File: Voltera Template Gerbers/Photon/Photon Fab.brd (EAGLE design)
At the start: 101.6 x 76.2 mm, 1 part

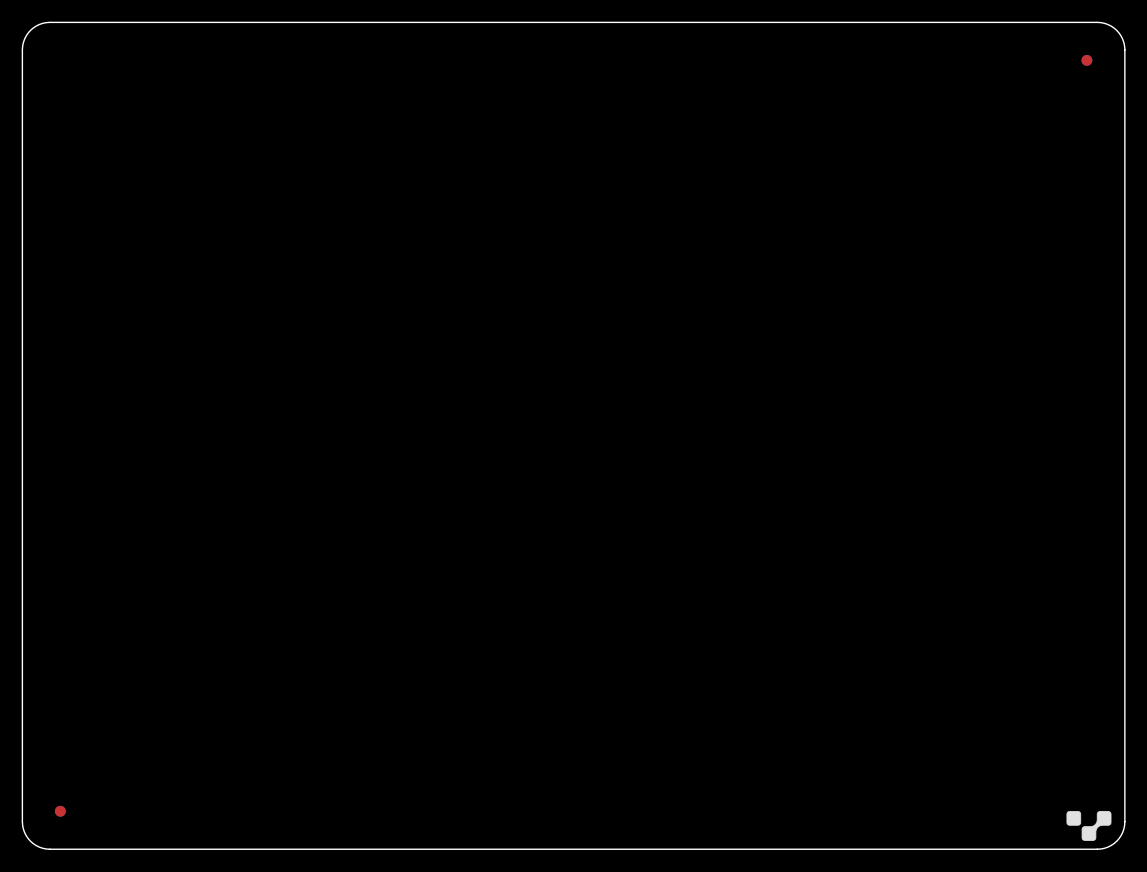
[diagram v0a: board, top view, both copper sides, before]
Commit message: Created FAB version for evertying, removed bad versions
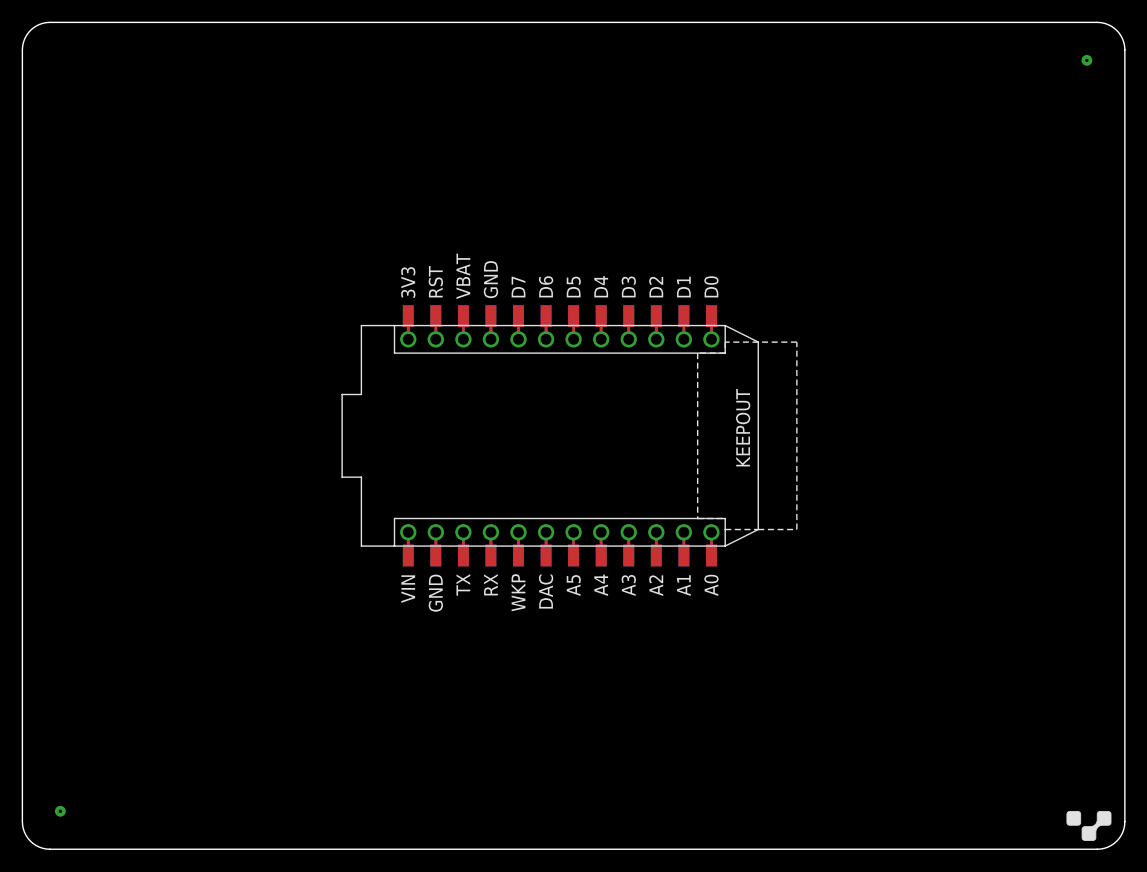
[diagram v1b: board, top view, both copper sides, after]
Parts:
- removed E$1: (no value), voltera_EAGLE_community_lib:3X4_BOARD
- added E$2: (no value), voltera_EAGLE_community_lib:PHOTON_RAW
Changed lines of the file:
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@@
 <?xml version="1.0" encoding="utf-8"?>
 <!DOCTYPE eagle SYSTEM "eagle.dtd">
-<eagle version="8.7.0">
+<eagle version="9.0.1">
 <drawing>
 <settings>
@@
 <setting verticaltext="up"/>
 </settings>
-<grid distance="0.05" unitdist="inch" unit="inch" style="lines" multiple="1" display="no" altdistance="0.025" altunitdist="inch" altunit="inch"/>
+<grid distance="0.05" unitdist="inch" unit="inch" style="lines" multiple="1" display="yes" altdistance="0.025" altunitdist="inch" altunit="inch"/>
 <layers>
 <layer number="1" name="Top" color="4" fill="1" visible="yes" active="yes"/>
@@
 </autorouter>
 <elements>
-<element name="E$1" library="voltera_EAGLE_community_lib" package="3X4_BOARD" value="" x="0" y="0"/>
+<element name="E$2" library="voltera_EAGLE_community_lib" package="PHOTON_RAW" value="" x="0" y="0"/>
 </elements>
 <signals>
